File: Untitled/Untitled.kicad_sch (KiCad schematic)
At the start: 50 parts, among them J1 Conn_01x02, J3 USB_C_Receptacle_USB2.0_14P, SW1 MX_SW_HS, SW2 MX_SW_HS, SW3 RST, SW4 RST, SW6 MX_SW_HS, SW7 MX_SW_HS, SW8 MX_SW_HS, SW9 MX_SW_HS, U1 nice_nano, U2 ATmega32U4-A, Y1 16MHz Crystal

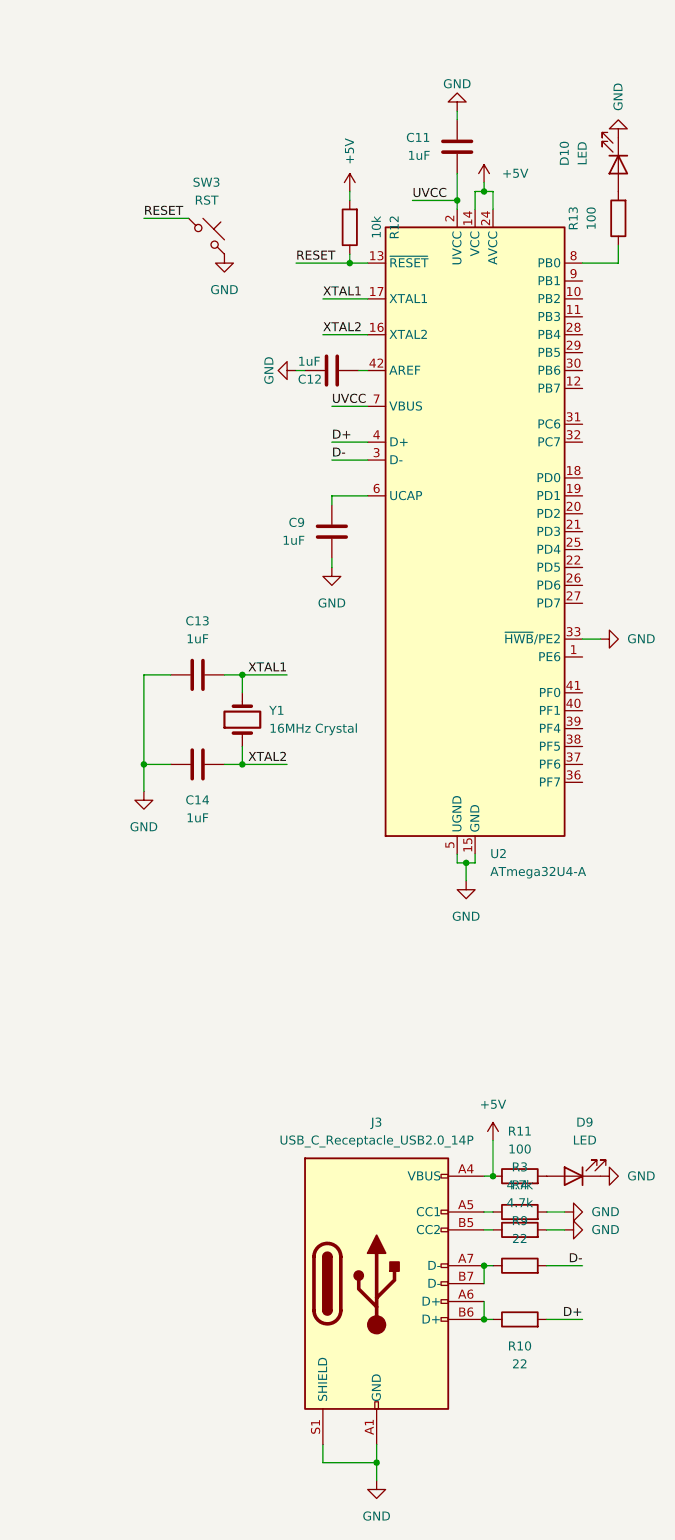
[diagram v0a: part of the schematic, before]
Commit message: idk
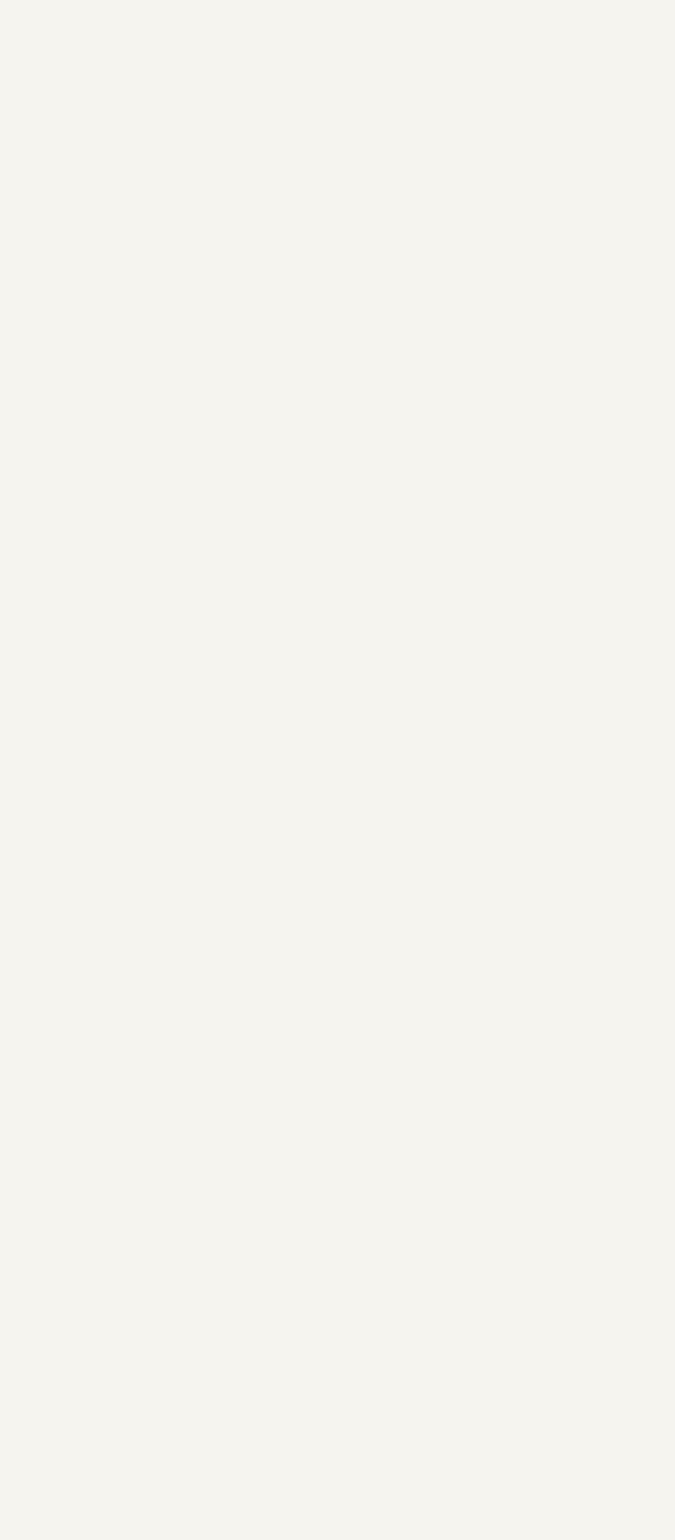
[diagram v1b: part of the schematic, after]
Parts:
- removed C11, C12, C13, C14, C9: 1uF, Capacitor_SMD:C_0805_2012Metric_Pad1.18x1.45mm_HandSolder, symbol Device:C
- removed D10, D9: LED, symbol Device:LED
- removed J3: USB_C_Receptacle_USB2.0_14P, symbol Connector:USB_C_Receptacle_USB2.0_14P
- removed R10, R9: 22, Resistor_SMD:R_0805_2012Metric_Pad1.20x1.40mm_HandSolder, symbol Device:R
- removed R11, R13: 100, Resistor_SMD:R_0805_2012Metric_Pad1.20x1.40mm_HandSolder, symbol Device:R
- removed R12: 10k, Resistor_SMD:R_0805_2012Metric_Pad1.20x1.40mm_HandSolder, symbol Device:R
- removed R3, R4: 4.7k, Resistor_SMD:R_0805_2012Metric_Pad1.20x1.40mm_HandSolder, symbol Device:R
- removed SW3: RST, Button_Switch_SMD:SW_Tactile_SPST_NO_Straight_CK_PTS636Sx25SMTRLFS, symbol Switch:SW_Push_45deg
- removed U2: ATmega32U4-A, Package_QFP:TQFP-44_10x10mm_P0.8mm, symbol MCU_Microchip_ATmega:ATmega32U4-A
- removed Y1: 16MHz Crystal, symbol Device:Crystal
